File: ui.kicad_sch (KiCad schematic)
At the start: 4 parts

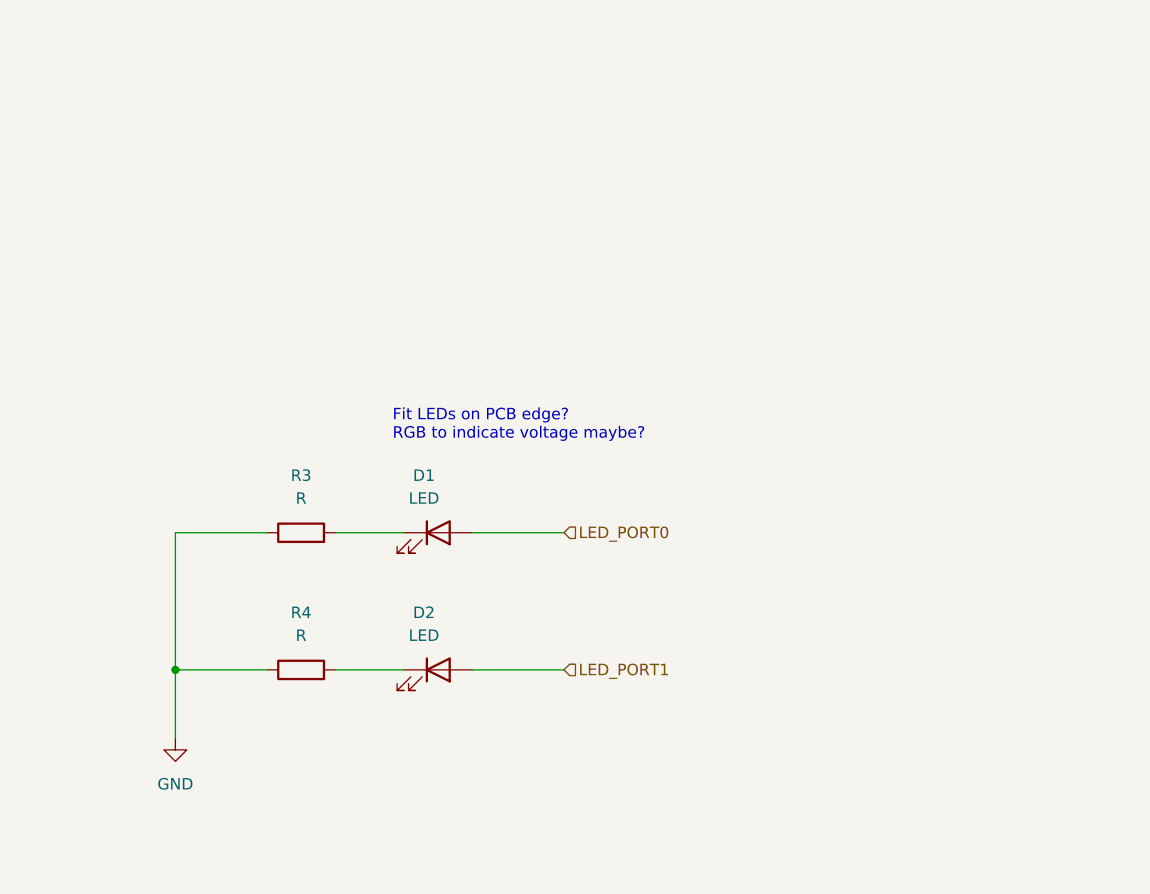
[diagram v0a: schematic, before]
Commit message: Wire more stuff
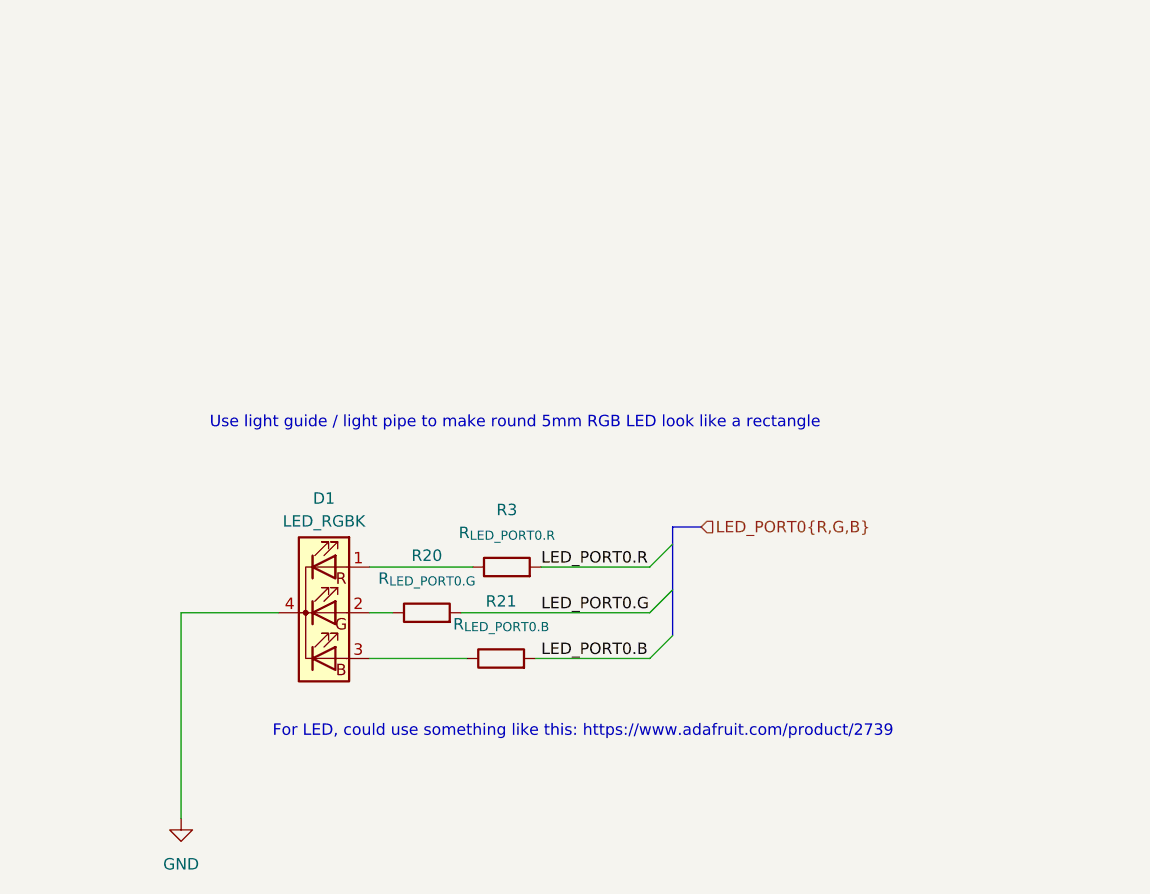
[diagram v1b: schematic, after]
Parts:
- removed D1, D2: LED, symbol Device:LED
- removed R4: R, symbol Device:R
- added D1: LED_RGBK, symbol Device:LED_RGBK
- added R20: R_{LED_PORT0.G}, symbol Device:R
- added R21: R_{LED_PORT0.B}, symbol Device:R
- R3: value R -> R_{LED_PORT0.R}
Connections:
- net GND: now also D1.4 (K); no longer R3.1
- net LED_PORT0.R: now reaches R3.2
- new net: D1.3 (BA), R21.1
- new net: D1.1 (RA), R3.1
- new net: D1.2 (GA), R20.1
- new net LED_PORT0.B: R21.2
- new net LED_PORT0.G: R20.2
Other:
- note added: "For LED, could use something like this: https://www.adafruit.com/product/2739"
- note added: "Use light guide / light pipe to make round 5mm RGB LED look like a rectangle"
- note removed: "Fit LEDs on PCB edge? RGB to indicate voltage maybe?"

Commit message: Whole bunch of changes to all kinds of things
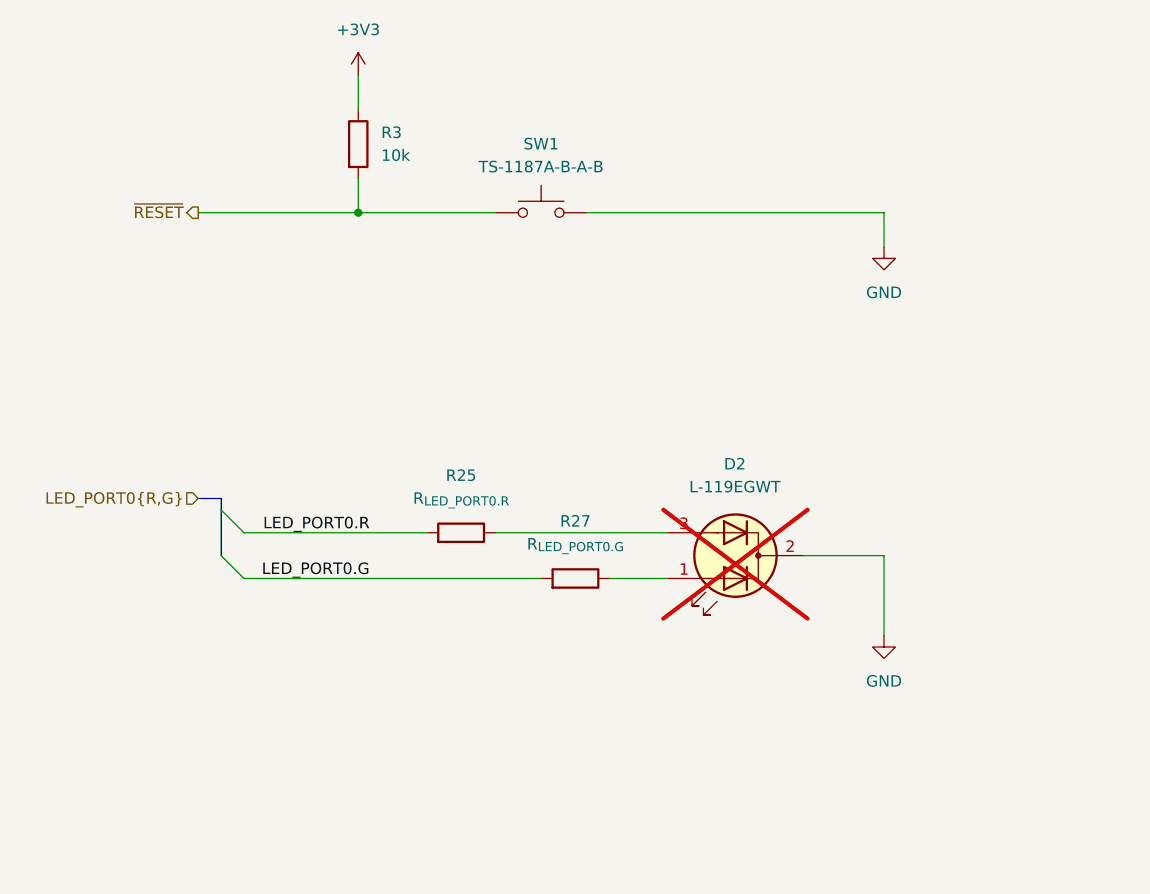
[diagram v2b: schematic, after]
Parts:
- removed D1: LED_RGBK, symbol Device:LED_RGBK
- removed R20: R_{LED_PORT0.G}, symbol Device:R
- removed R21: R_{LED_PORT0.B}, symbol Device:R
- added D2: L-119EGWT, symbol Device:LED_Dual_AKA
- added R25: R_{LED_PORT0.R}, symbol Device:R
- added R27: R_{LED_PORT0.G}, symbol Device:R
- added SW1: TS-1187A-B-A-B, symbol Switch:SW_Push
- R3: value R_{LED_PORT0.R} -> 10k
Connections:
- net GND: now also D2.2 (K), SW1.2
- net LED_PORT0.G: now also R27.2
- net LED_PORT0.R: now also R25.2; no longer R3.2
- net +3V3: now reaches R3.1
- new net: D2.3 (A2), R25.1
- new net: D2.1 (A1), R27.1
- new net ~{RESET}: R3.2, SW1.1
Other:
- note removed: "For LED, could use something like this: https://www.adafruit.com/product/2739"
- note removed: "Use light guide / light pipe to make round 5mm RGB LED look like a rectangle"
